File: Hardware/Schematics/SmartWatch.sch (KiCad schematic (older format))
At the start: 93 parts, among them J1 PIC32_ICSP, J2 USB_C_Receptacle, M1 Motor_DC, Q1 2N7000, Q2 Photo_NPN, SW1 SW_Push, SW2 SW_Push, U1 nRF8001, U2 PIC32MZ2048EFG064, U3 LSM303AGR, U4 STMPE811, U5 BQ25010, Y1 Crystal_GND24, Y2 64MHz, Y3 32.768kHz

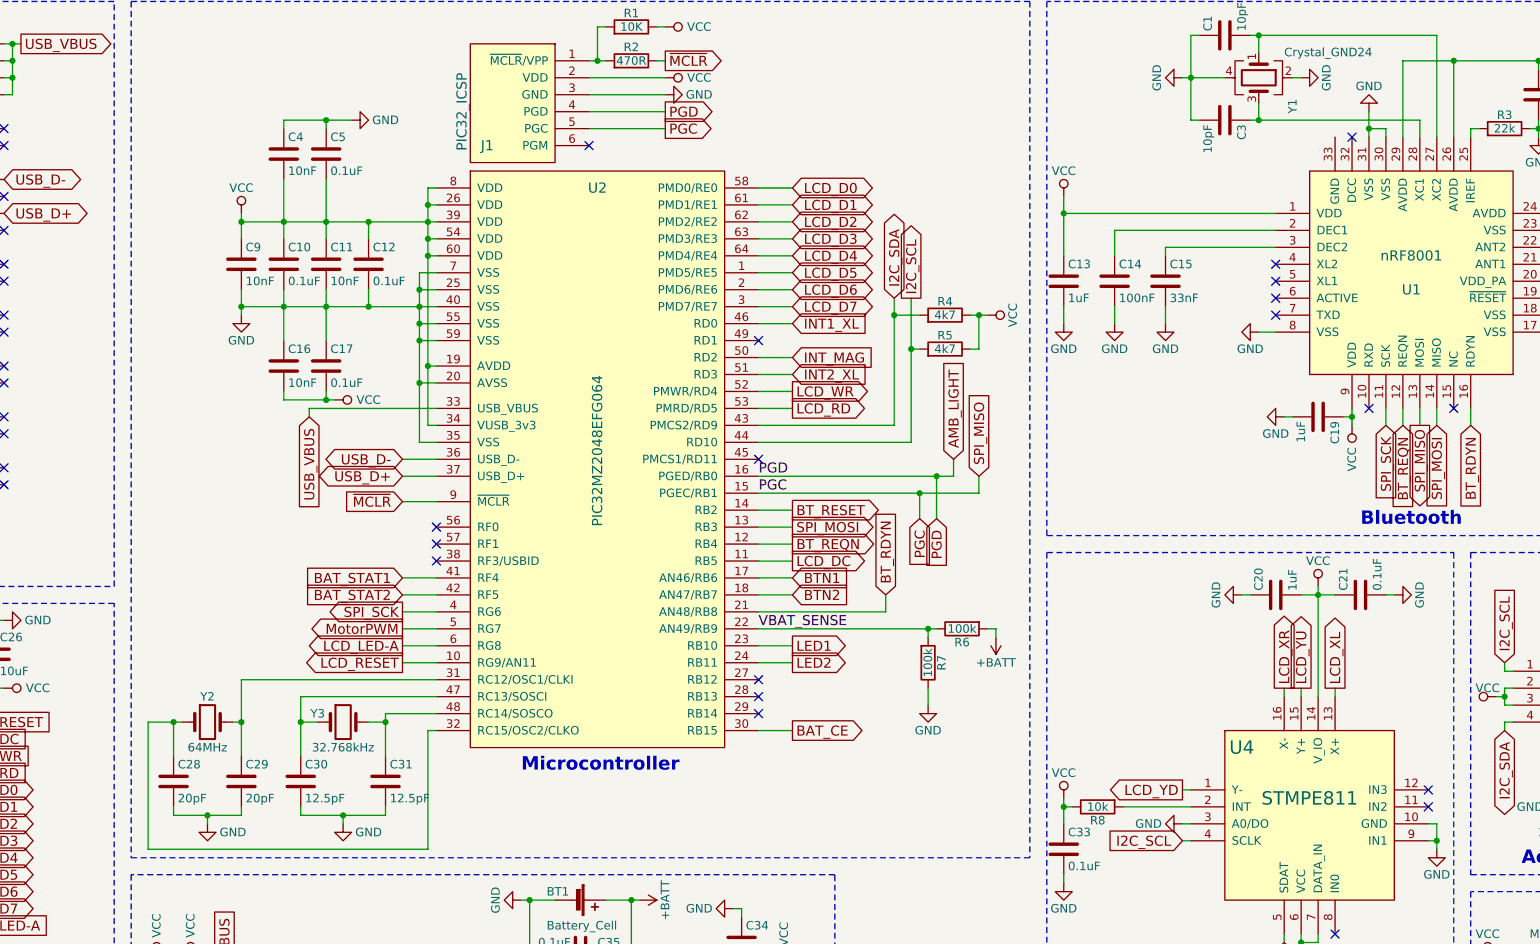
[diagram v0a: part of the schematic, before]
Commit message: PCB
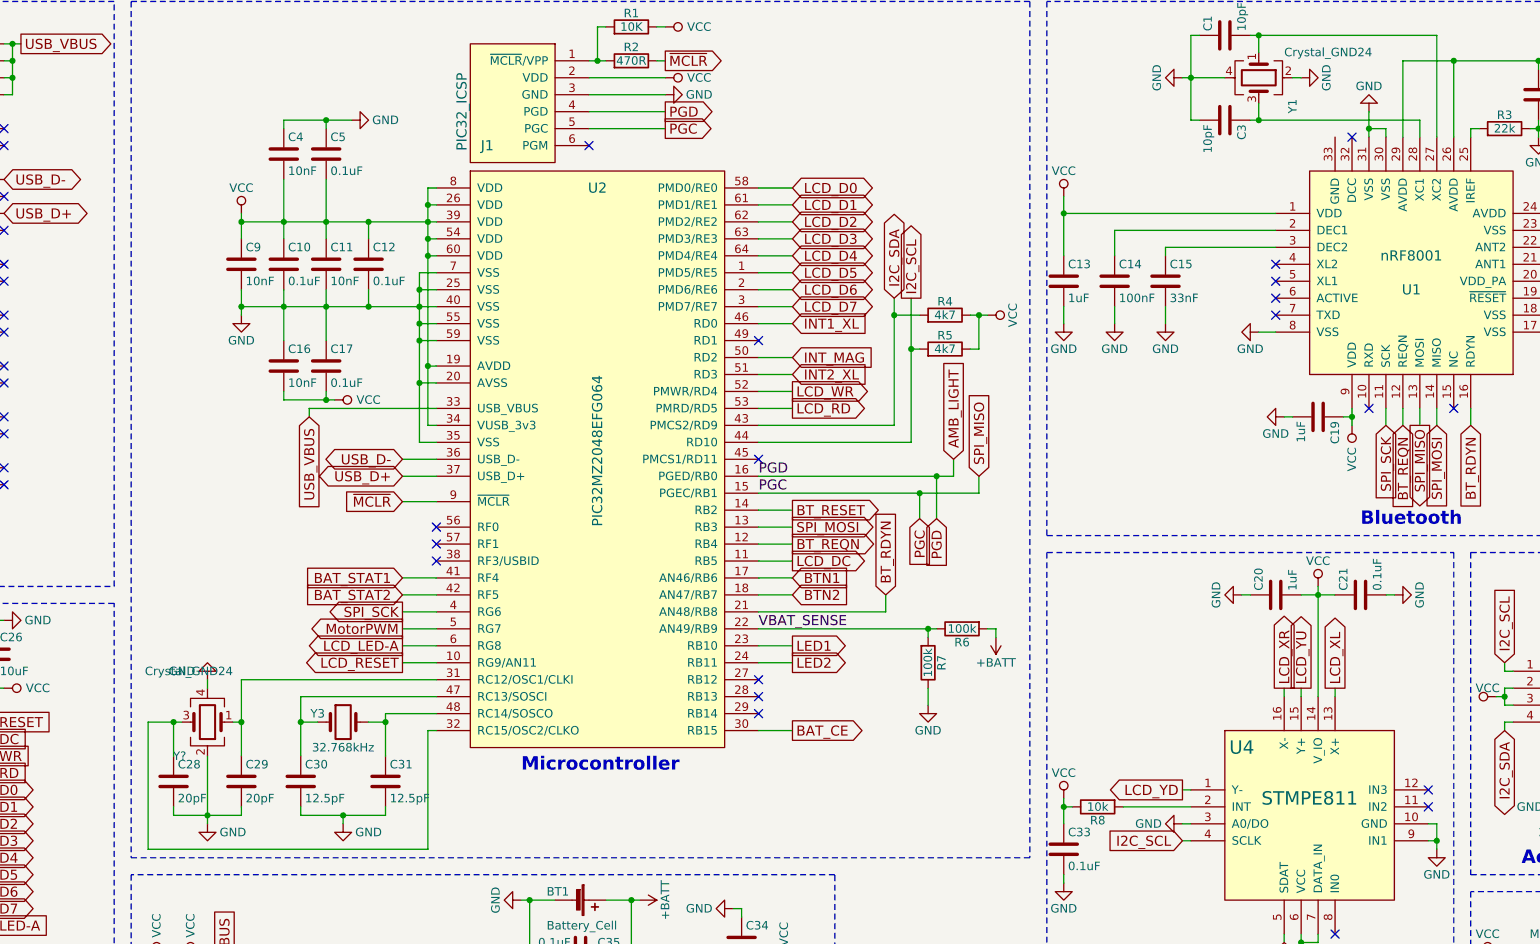
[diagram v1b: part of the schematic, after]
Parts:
- removed Y2: 64MHz, 2450AT18A100E:CX2520DB16000F0FDFC1, symbol Crystal
- added Y?: Crystal_GND24, 2450AT18A100E:CX2520DB16000F0FDFC1, symbol Crystal_GND24
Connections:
- net GND: now also Y?.2, Y?.4
- net at C29.1, U2.31 (RC12/OSC1/CLKI): now also Y?.1
- net at C28.1, U2.32 (RC15/OSC2/CLKO): now also Y?.3
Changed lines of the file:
@@
 $EndComp
 $Comp
-L Crystal Y2
-U 1 1 5A2813FF
-P 4900 6000
-F 0 "Y2" H 4900 6150 50  0000 C CNN
-F 1 "64MHz" H 4900 5850 50  0000 C CNN
-F 2 "2450AT18A100E:CX2520DB16000F0FDFC1" H 4900 6000 50  0001 C CNN
-F 3 "" H 4900 6000 50  0001 C CNN
-	1    4900 6000
-	1    0    0    -1
-$EndComp
-$Comp
 L C C28
 U 1 1 5A281E18
@@
 	4700 6550 4700 6500
 Wire Wire Line
-	4900 6550 4900 6600
+	4900 6200 4900 6600
 Wire Wire Line
 	4700 6550 5100 6550
@@
 	12050 2450 12050 2550
 Wire Wire Line
-	11050 2450 12050 2450
-Connection ~ 11100 2450
-Wire Wire Line
-	11100 2350 11100 2450
-Wire Wire Line
-	11100 2050 11100 1950
-Wire Wire Line
-	11050 1950 12150 1950
-Wire Wire Line
 	12150 1950 12150 2550
-Connection ~ 11100 1950
 Wire Wire Line
 	10700 1950 10700 2450
@@
 Wire Wire Line
 	11450 7300 11450 7250
+Wire Wire Line
+	12050 2450 11050 2450
+Wire Wire Line
+	11050 1950 12150 1950
+Wire Wire Line
+	11100 2050 11100 1950
+Connection ~ 11100 1950
+Wire Wire Line
+	11100 2350 11100 2450
+Connection ~ 11100 2450
+$Comp
+L Crystal_GND24 Y?
+U 1 1 5A615765
+P 4900 6000
+F 0 "Y?" H 5025 6200 50  0000 L CNN
+F 1 "Crystal_GND24" H 4750 5700 50  0000 L CNN
+F 2 "2450AT18A100E:CX2520DB16000F0FDFC1" H 4900 6000 50  0001 C CNN
+F 3 "" H 4900 6000 50  0001 C CNN
+	1    4900 6000
+	-1   0    0    1
+$EndComp
+$Comp
+L GND #PWR?
+U 1 1 5A6162C7
+P 4900 5750
+F 0 "#PWR?" H 4900 5500 50  0001 C CNN
+F 1 "GND" H 5050 5700 50  0000 C CNN
+F 2 "" H 4900 5750 50  0001 C CNN
+F 3 "" H 4900 5750 50  0001 C CNN
+	1    4900 5750
+	-1   0    0    1
+$EndComp
+Wire Wire Line
+	4900 5800 4900 5750
 $EndSCHEMATC
